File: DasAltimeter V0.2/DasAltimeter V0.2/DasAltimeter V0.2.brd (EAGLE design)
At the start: 38.9 x 21.6 mm, 53 parts, among them IC1 BMI055, U1 ATSAMD21G-A, U2 3.3V/150mA, U3 MS5803-14BA, U4 ADXL193, X1 22-23-2041, X2 22-23-2041

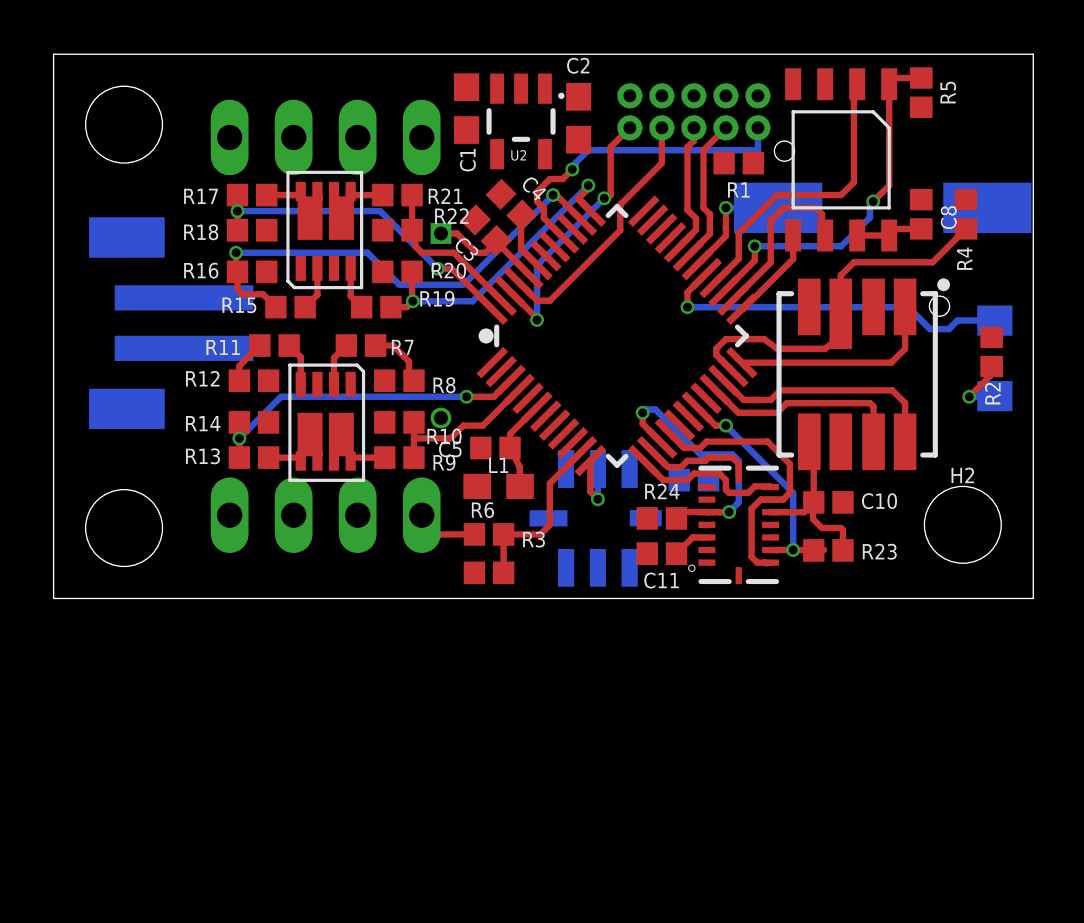
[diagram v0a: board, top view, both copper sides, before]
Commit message: playing with mini altimeter idea
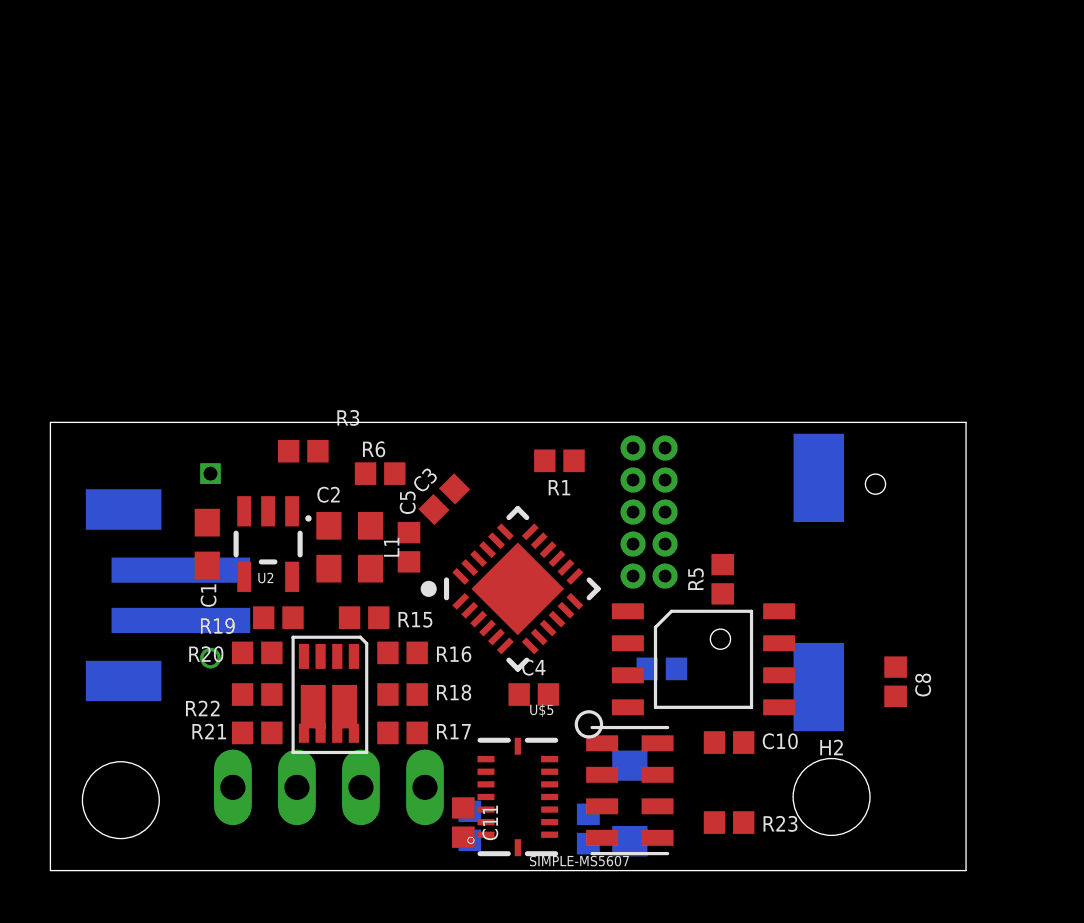
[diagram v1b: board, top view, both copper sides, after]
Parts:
- removed C9: 0.1uF, SparkFun-Capacitors:0402
- removed H1: STAND-OFFTIGHT, SparkFun-Hardware:STAND-OFF-TIGHT
- removed R10, R14: 27k, SparkFun-Resistors:0402
- removed R11, R7: 100, SparkFun-Resistors:0402
- removed R12, R8: 3.3k, SparkFun-Resistors:0402
- removed R13, R9: 100k, SparkFun-Resistors:0402
- removed U$3: SI7232DN, SaL-lib1:SI7232DN
- removed U1: ATSAMD21G-A, SparkFun-IC-Microcontroller:TQFP-48
- removed U3: MS5803-14BA, SparkFun-Sensors:MS5803
- removed U4: ADXL193, SparkFun-Sensors:LCC-8
- removed X1: 22-23-2041, con-molex:22-23-2041
- added U$2: ATSAMD10D, SaL-lib1:ATSAMD10D
- added U$5: SIMPLE-MS5607, MS5607:MS5607
- C3: value 0.1uF -> 100nF
- C5: value 0.1uF -> 4.7uF
- moved X2 25.8 mm to (10.9, -7.49), turned to 0 degrees
- moved R2 24.8 mm to (21.2, -9.14), flipped to the bottom
- moved D2 22.8 mm to (22.9, -8.13)
- moved R17 22.2 mm to (13.8, -5.33), turned to 0 degrees
- moved R21 22.0 mm to (8.08, -5.33), turned to 0 degrees
- moved R4 21.7 mm to (24.1, -2.79), flipped to the bottom, turned to 0 degrees
- moved MEM 21.0 mm to (25.8, -3.05), turned to 0 degrees
- moved R5 20.8 mm to (26.5, 0.76), turned to 90 degrees
- moved C1 20.1 mm to (6.10, 2.16)
- moved C2 19.7 mm to (10.9, 2.03)
- moved U2 19.5 mm to (8.51, 2.16)
- moved C4 19.5 mm to (19.1, -3.81), turned to 0 degrees
- moved R18 19.4 mm to (13.8, -3.81), turned to 180 degrees
- moved R22 19.2 mm to (8.08, -3.81), turned to 180 degrees
- moved C8 18.6 mm to (33.4, -3.30)
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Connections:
- removed net FET_C: R9.1, U$3.7, U$3.8, U$3.9, X1.2
- removed net FET_D: R13.2, U$3.10, U$3.5, U$3.6, X1.3
- removed net FIRE_C: R7.2, R8.1, U1.34
- removed net FIRE_D: R11.1, R12.2, U1.33
- removed net N$3: C4.1, U1.43
- removed net N$8: R11.2, U$3.4
- removed net SENSE_C: R10.1, R9.2, U1.4
- removed net SENSE_D: R13.1, R14.2, U1.3
- removed net SPI0_MISO: IC1.10, IC1.15, U1.16
- removed net SPI0_MOSI: IC1.9, U1.13
- removed net SPI0_SCK: IC1.8, U1.14
- removed net SPI2_MISO: U1.22, U3.8
- removed net SPI2_MOSI: U1.21, U3.7
- removed net SPI2_SCK: U1.24, U3.1
- net !RESET: now also U$2.18; no longer U1.40
- net 3.3V: now also C4.1; no longer C3.1, C9.1, U1.17, U1.36, U1.44, U3.5, U4.P$7, U4.P$8
- net ACCELX: now also U$2.6; no longer U1.12, U4.P$6
- net BUZZER: now also U$2.10; no longer U1.30
- net CS_ACCEL: now also U$2.11; no longer U1.19
- net CS_BARO: now also U$2.17, U$5.5; no longer U1.23, U3.3
- net CS_GYRO: now also U$2.12; no longer U1.15
- net CS_MEM: now also U$2.13; no longer U1.27
- net FIRE_A: now also U$2.8; no longer U1.38
- net FIRE_B: now also U$2.7; no longer U1.37
- net GND: now also U$2.23, U$5.3; no longer C4.2, C9.2, R10.2, R12.1, R14.1, R8.2, U$3.1, U$3.3, U1.18, U1.35, U1.42, U1.5, U3.2, U3.6, U4.P$3
- net LED: now also U$2.9; no longer U1.29
- net N$1: now also C4.2, U$5.1; no longer R7.1, U$3.2
- net N$4: now also C3.1, U$2.24; no longer U1.6
- net RX: now also U$2.22; no longer U1.32
- net SENSE_A: now also U$2.1; no longer U1.48
- net SENSE_B: now also U$2.2; no longer U1.47
- net SENSE_BAT: now also U$2.5; no longer U1.11
- net SPI1_MISO: now also IC1.10, IC1.15, U$2.14; no longer U1.28
- net SPI1_MOSI: now also IC1.9, U$2.15; no longer U1.25
- net SPI1_SCK: now also IC1.8, U$2.16; no longer U1.26
- net SWCLK: now also U$2.19; no longer U1.45
- net SWDIO: now also U$2.20; no longer U1.46
- net TX: now also U$2.21; no longer U1.31
- net VCC: no longer X1.1, X1.4
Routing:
- net FIRE_A: track 19.4 -> 0.00 mm, vias 2 -> 0
- net 3.3V: track 15.8 -> 0.00 mm
- net CS_BARO: track 14.7 -> 0.00 mm
- net CS_MEM: track 14.4 -> 0.00 mm, vias 2 -> 0
- net LED: track 14.3 -> 0.00 mm, vias 1 -> 0
- net SENSE_A: track 13.1 -> 0.00 mm, vias 2 -> 0
- net SENSE_D: track 13.1 -> 0.00 mm, vias 2 -> 0
- net !RESET: track 12.7 -> 0.00 mm, vias 1 -> 0
- net FIRE_B: track 12.4 -> 0.00 mm, vias 2 -> 0
- net SPI1_MISO: track 12.2 -> 0.00 mm
- net SPI0_MISO: track 11.1 -> 0.00 mm
- net SWDIO: track 10.8 -> 0.00 mm, vias 2 -> 0
- net CS_GYRO: track 10.6 -> 0.00 mm, vias 2 -> 0
- net SWCLK: track 10.2 -> 0.00 mm
- net CS_ACCEL: track 9.99 -> 0.00 mm, vias 2 -> 0
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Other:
- board size 38.9 x 21.6 mm -> 36.3 x 17.8 mm
